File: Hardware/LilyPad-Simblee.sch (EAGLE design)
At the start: 37 parts, among them U1 MIC5219 3.3V, U2 MCP73831, U3 RFD77101

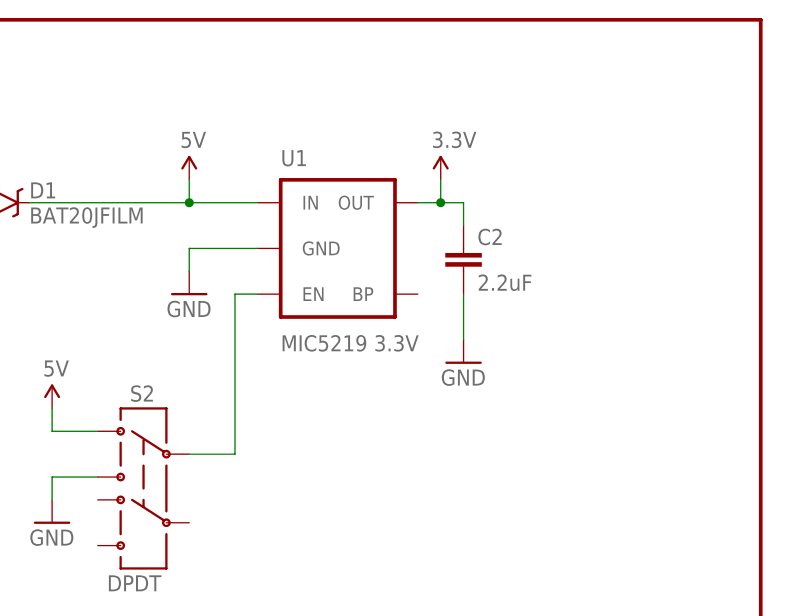
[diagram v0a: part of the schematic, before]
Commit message: Release
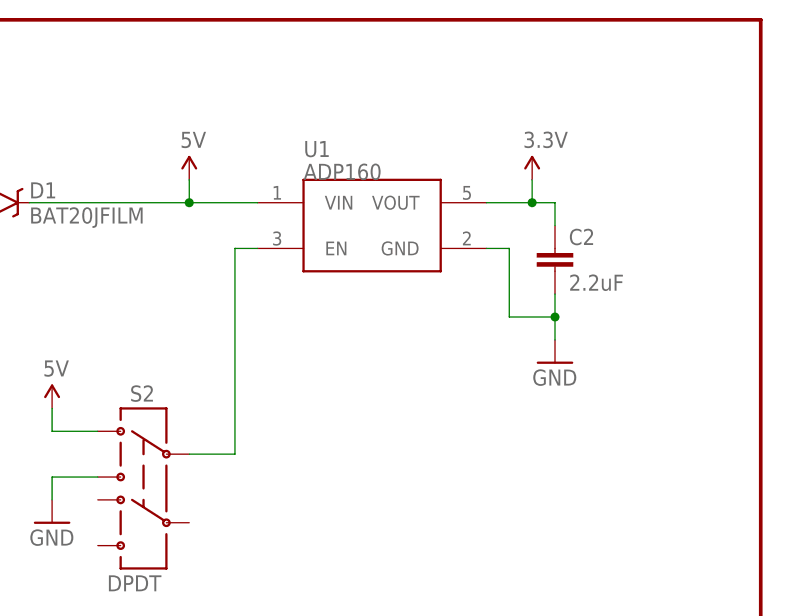
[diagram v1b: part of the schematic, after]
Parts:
- U1: value MIC5219 3.3V -> ADP160; device SparkFun-PowerIC:V_REG_MIC52193.3V -> SparkFun-PowerIC:ADP160
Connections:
- net 3.3V: now also U1.VOUT; no longer U1.OUT
- net 5V: now also U1.VIN; no longer U1.IN
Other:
- moved on the sheet: C2
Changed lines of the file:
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@@
 <part name="A5/19" library="LilyPad-Wearables" deviceset="SEWTAP" device="9"/>
 <part name="U$4" library="LilyPad-Wearables" deviceset="SEWTAP" device="9"/>
-<part name="GND3" library="SparkFun" deviceset="GND" device=""/>
 <part name="GND9" library="SparkFun" deviceset="GND" device=""/>
 <part name="JP2" library="SparkFun-Connectors" deviceset="ARDUINO_SERIAL_PROGRAM" device="SMD">
@@
 <part name="SUPPLY9" library="SparkFun-Aesthetics" deviceset="V_BATT" device=""/>
 <part name="C2" library="SparkFun-Capacitors" deviceset="2.2UF-10V-20%(0603)" device="" value="2.2uF"/>
-<part name="U1" library="SparkFun-PowerIC" deviceset="V_REG_MIC5219" device="3.3V" value="MIC5219 3.3V"/>
 <part name="D1" library="SparkFun-DiscreteSemi" deviceset="BAT20JFILM" device="" value="BAT20JFILM"/>
 <part name="SUPPLY10" library="SparkFun-Aesthetics" deviceset="5V" device=""/>
@@
 <part name="U$1" library="LilyPad-Wearables" deviceset="LOGO-LP" device="L"/>
 <part name="U$2" library="LilyPad-Wearables" deviceset="LOGO-LP" device="LP"/>
+<part name="U1" library="SparkFun-PowerIC" deviceset="ADP160" device="" value="ADP160"/>
 </parts>
 <sheets>
@@
 <instance part="A5/19" gate="G$1" x="187.96" y="58.42" smashed="yes"/>
 <instance part="U$4" gate="G$1" x="187.96" y="66.04" smashed="yes"/>
-<instance part="GND3" gate="1" x="185.42" y="154.94"/>
 <instance part="GND9" gate="1" x="48.26" y="55.88"/>
 <instance part="JP2" gate="G$1" x="175.26" y="101.6" rot="R180">
@@
 <instance part="SUPPLY1" gate="G$1" x="30.48" y="104.14"/>
 <instance part="SUPPLY2" gate="G$1" x="40.64" y="99.06"/>
-<instance part="GND4" gate="1" x="215.9" y="147.32"/>
-<instance part="SUPPLY3" gate="G$1" x="213.36" y="167.64"/>
+<instance part="GND4" gate="1" x="226.06" y="147.32"/>
+<instance part="SUPPLY3" gate="G$1" x="223.52" y="167.64"/>
 <instance part="SUPPLY4" gate="G$1" x="15.24" y="43.18"/>
 <instance part="SUPPLY6" gate="G$1" x="167.64" y="109.22"/>
@@
 <instance part="SUPPLY8" gate="G$1" x="63.5" y="149.86"/>
 <instance part="SUPPLY9" gate="G$1" x="149.86" y="167.64"/>
-<instance part="C2" gate="G$1" x="215.9" y="157.48"/>
-<instance part="U1" gate="G$1" x="203.2" y="160.02"/>
+<instance part="C2" gate="G$1" x="226.06" y="157.48"/>
 <instance part="D1" gate="G$1" x="165.1" y="165.1"/>
 <instance part="SUPPLY10" gate="G$1" x="185.42" y="167.64"/>
@@
 <instance part="U$1" gate="G$1" x="236.22" y="17.78"/>
 <instance part="U$2" gate="G$1" x="236.22" y="17.78"/>
+<instance part="U1" gate="G$1" x="205.74" y="162.56"/>
 </instances>
 <busses>
@@
 </segment>
 <segment>
-<pinref part="GND3" gate="1" pin="GND"/>
-<wire x1="185.42" y1="157.48" x2="185.42" y2="160.02" width="0.1524" layer="91"/>
-<pinref part="U1" gate="G$1" pin="GND"/>
-<wire x1="185.42" y1="160.02" x2="193.04" y2="160.02" width="0.1524" layer="91"/>
-</segment>
-<segment>
 <pinref part="GND5" gate="1" pin="GND"/>
 <wire x1="170.18" y1="132.08" x2="170.18" y2="134.62" width="0.1524" layer="91"/>
@@
 <pinref part="GND4" gate="1" pin="GND"/>
 <pinref part="C2" gate="G$1" pin="2"/>
-<wire x1="215.9" y1="149.86" x2="215.9" y2="154.94" width="0.1524" layer="91"/>
+<wire x1="226.06" y1="149.86" x2="226.06" y2="152.4" width="0.1524" layer="91"/>
+<wire x1="226.06" y1="152.4" x2="226.06" y2="154.94" width="0.1524" layer="91"/>
+<wire x1="220.98" y1="160.02" x2="220.98" y2="152.4" width="0.1524" layer="91"/>
+<wire x1="220.98" y1="152.4" x2="226.06" y2="152.4" width="0.1524" layer="91"/>
+<junction x="226.06" y="152.4"/>
+<pinref part="U1" gate="G$1" pin="GND"/>
+<wire x1="218.44" y1="160.02" x2="220.98" y2="160.02" width="0.1524" layer="91"/>
 </segment>
 <segment>
@@
 </segment>
 <segment>
-<pinref part="U1" gate="G$1" pin="OUT"/>
 <pinref part="SUPPLY3" gate="G$1" pin="3.3V"/>
-<wire x1="210.82" y1="165.1" x2="213.36" y2="165.1" width="0.1524" layer="91"/>
-<wire x1="213.36" y1="165.1" x2="213.36" y2="167.64" width="0.1524" layer="91"/>
+<wire x1="223.52" y1="165.1" x2="223.52" y2="167.64" width="0.1524" layer="91"/>
 <pinref part="C2" gate="G$1" pin="1"/>
-<wire x1="213.36" y1="165.1" x2="215.9" y2="165.1" width="0.1524" layer="91"/>
-<wire x1="215.9" y1="165.1" x2="215.9" y2="162.56" width="0.1524" layer="91"/>
-<junction x="213.36" y="165.1"/>
+<wire x1="223.52" y1="165.1" x2="226.06" y2="165.1" width="0.1524" layer="91"/>
+<wire x1="226.06" y1="165.1" x2="226.06" y2="162.56" width="0.1524" layer="91"/>
+<pinref part="U1" gate="G$1" pin="VOUT"/>
+<wire x1="218.44" y1="165.1" x2="223.52" y2="165.1" width="0.1524" layer="91"/>
+<junction x="223.52" y="165.1"/>
 </segment>
 <segment>
@@
 <segment>
 <wire x1="193.04" y1="165.1" x2="185.42" y2="165.1" width="0.1524" layer="91"/>
-<pinref part="U1" gate="G$1" pin="IN"/>
 <pinref part="D1" gate="G$1" pin="C"/>
 <wire x1="167.64" y1="165.1" x2="185.42" y2="165.1" width="0.1524" layer="91"/>
@@
 <wire x1="185.42" y1="167.64" x2="185.42" y2="165.1" width="0.1524" layer="91"/>
 <junction x="185.42" y="165.1"/>
+<pinref part="U1" gate="G$1" pin="VIN"/>
 </segment>
 <segment>
@@
 <pinref part="S2" gate="G$1" pin="2"/>
 <wire x1="185.42" y1="137.16" x2="190.5" y2="137.16" width="0.1524" layer="91"/>
-<wire x1="190.5" y1="137.16" x2="190.5" y2="154.94" width="0.1524" layer="91"/>
+<wire x1="190.5" y1="137.16" x2="190.5" y2="160.02" width="0.1524" layer="91"/>
 <pinref part="U1" gate="G$1" pin="EN"/>
-<wire x1="190.5" y1="154.94" x2="193.04" y2="154.94" width="0.1524" layer="91"/>
-</segment>
-</net>
+<wire x1="190.5" y1="160.02" x2="193.04" y2="160.02" width="0.1524" layer="91"/>
+</segment>
+</net>
